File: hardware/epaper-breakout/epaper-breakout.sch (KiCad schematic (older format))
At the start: 87 parts, among them J1 XF2M-3315-1A, J2 C10418, J3 Conn_02x06_Counter_Clockwise, J4 ED060SC4, Q1 AO3401A, Q2 AO3401A, Q3 MMBT3904, Q4 MMBT3904, Q5 AO3401A, Q6 MMBT3904, U1 MCP1700-3302E_SOT23, U10 ED060SC7, U11 TP4056, U12 FS312F-G, U13 FS8205A, U2 LT1945, U3 LT1945, U4 CH340G, U5 ESP32-WROVER, U6 ED060XC5, U7 LM358, U8 74HC4094-normal, U9 MCP9700AT-ETT, Y1 Crystal_GND2

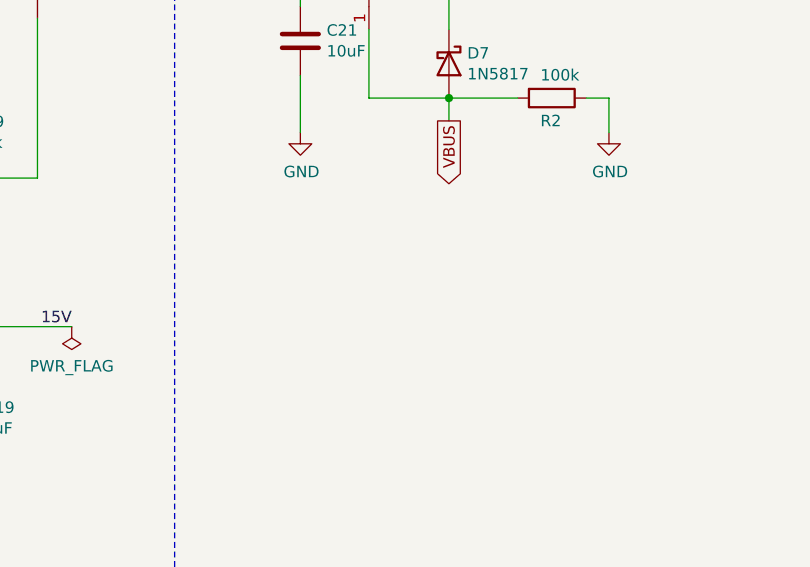
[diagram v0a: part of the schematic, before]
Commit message: more routing
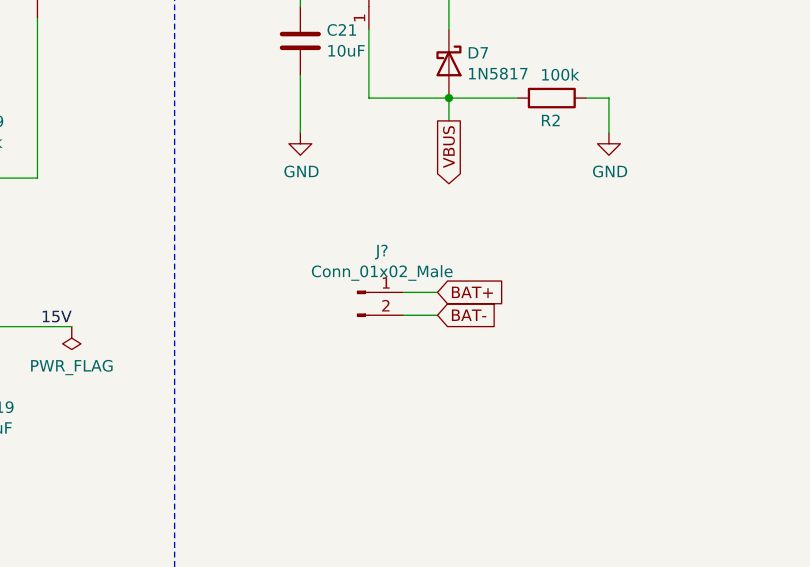
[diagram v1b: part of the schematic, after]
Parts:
- added J?: Conn_01x02_Male, Connector_PinHeader_2.54mm:PinHeader_1x02_P2.54mm_Vertical, symbol Connector:Conn_01x02_Male
- D7: footprint Diode_THT:D_DO-41_SOD81_P10.16mm_Horizontal -> Diode_SMD:D_SOD-123
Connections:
- net BAT+: now also J?.1 (Pin_1)
- net BAT-: now also J?.2 (Pin_2)
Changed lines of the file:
@@
 F 0 "D7" V 6104 5830 50  0000 L CNN
 F 1 "1N5817" V 6195 5830 50  0000 L CNN
-F 2 "Diode_THT:D_DO-41_SOD81_P10.16mm_Horizontal" H 6150 5575 50  0001 C CNN
+F 2 "Diode_SMD:D_SOD-123" H 6150 5575 50  0001 C CNN
 F 3 "http://www.vishay.com/docs/88525/1n5817.pdf" H 6150 5750 50  0001 C CNN
 	1    6150 5750
@@
 Wire Wire Line
 	7600 4250 7900 4250
+$Comp
+L Connector:Conn_01x02_Male J?
+U 1 1 655CB8A7
+P 5750 6750
+F 0 "J?" H 5858 6931 50  0000 C CNN
+F 1 "Conn_01x02_Male" H 5858 6840 50  0000 C CNN
+F 2 "Connector_PinHeader_2.54mm:PinHeader_1x02_P2.54mm_Vertical" H 5750 6750 50  0001 C CNN
+F 3 "~" H 5750 6750 50  0001 C CNN
+	1    5750 6750
+	1    0    0    -1
+$EndComp
+Text GLabel 6100 6750 2    50   Input ~ 0
+BAT+
+Text GLabel 6100 6850 2    50   Input ~ 0
+BAT-
+Wire Wire Line
+	5950 6750 6100 6750
+Wire Wire Line
+	6100 6850 5950 6850
 $EndSCHEMATC
